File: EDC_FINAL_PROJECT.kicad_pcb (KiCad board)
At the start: 2 copper layers, 88.9 x 50.8 mm, 31 parts, among them J1 Screw_Terminal_01x02, J2 Screw_Terminal_01x03, SW1 SW_Push_DPDT, U1 LM317_TO-220, U2 LM337_TO220

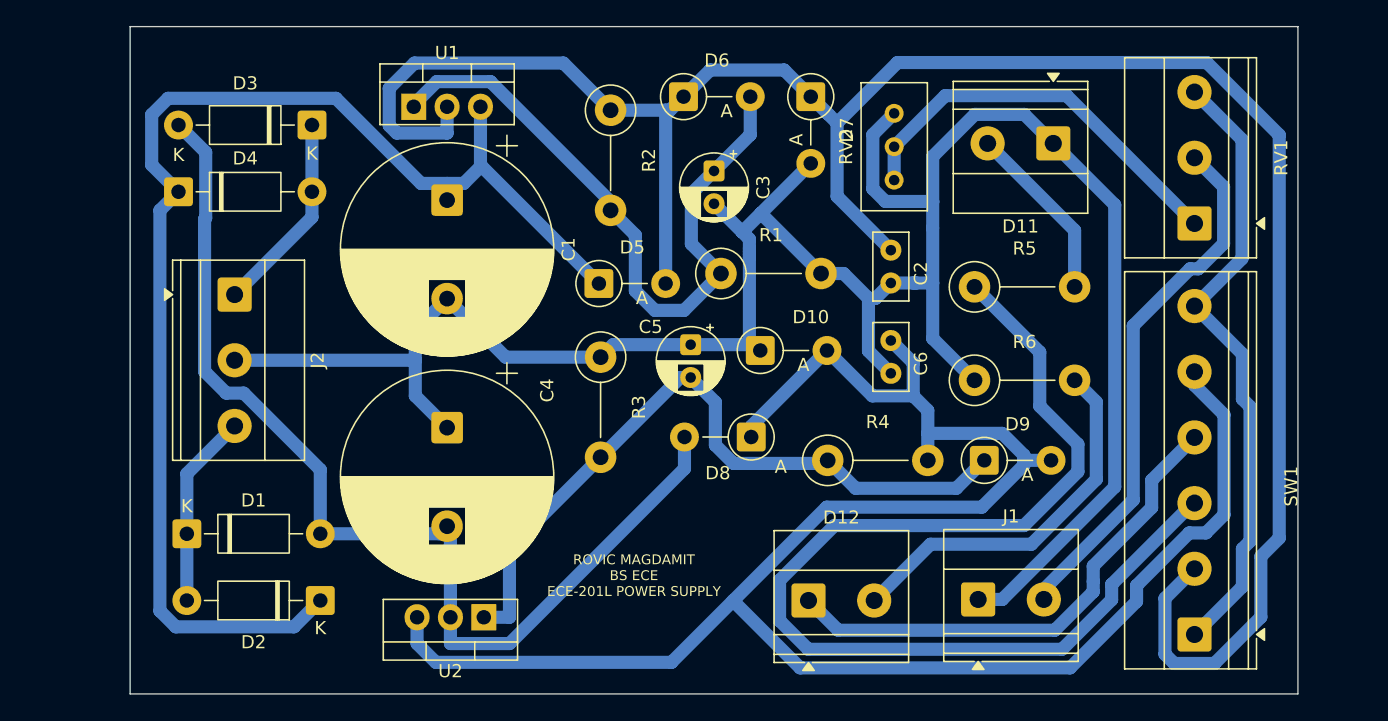
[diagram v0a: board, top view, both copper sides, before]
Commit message: 10.17.2025
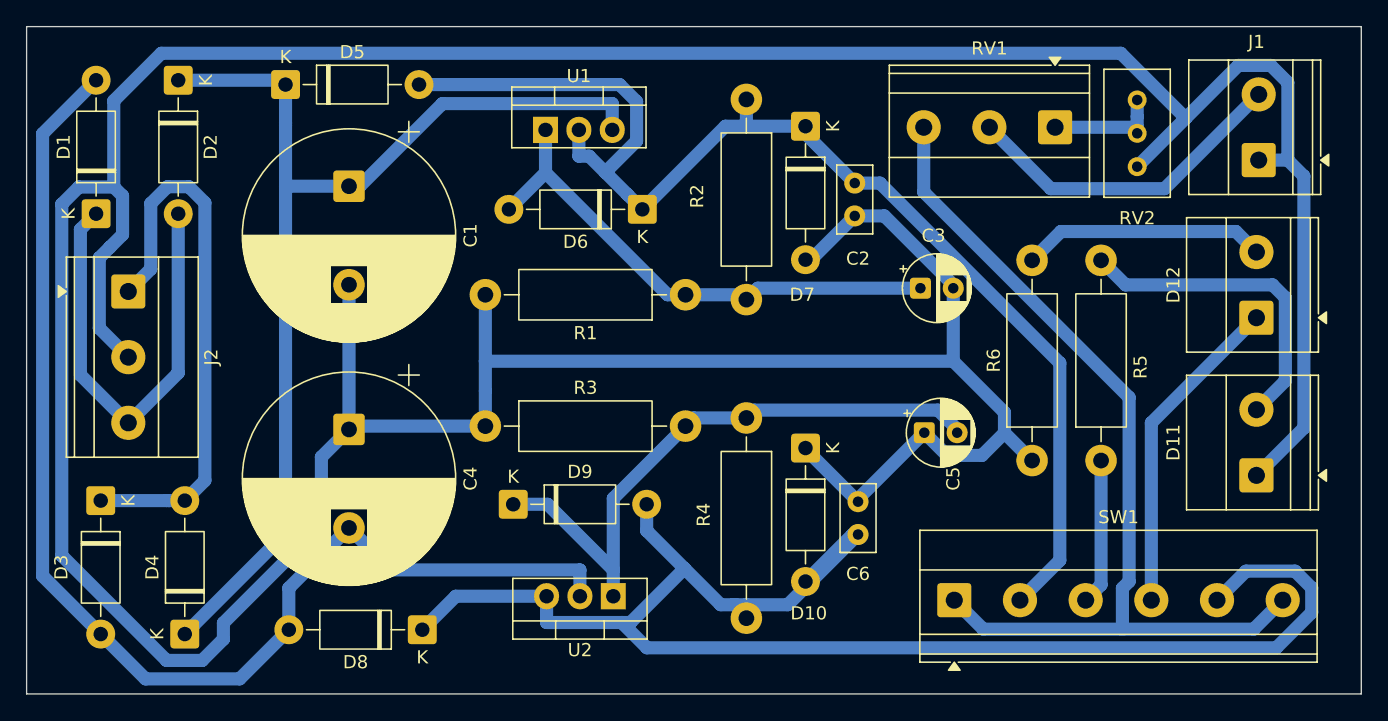
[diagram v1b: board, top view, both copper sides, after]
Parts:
- D10, D5, D6, D7, D8, D9: footprint Diode_THT:D_DO-41_SOD81_P5.08mm_Vertical_AnodeUp -> Diode_THT:D_DO-41_SOD81_P10.16mm_Horizontal
- R1, R2, R3, R4, R5, R6: footprint Resistor_THT:R_Axial_DIN0411_L9.9mm_D3.6mm_P7.62mm_Vertical -> Resistor_THT:R_Axial_DIN0411_L9.9mm_D3.6mm_P15.24mm_Horizontal
- moved D2 41.1 mm to (103.6, 77.2), turned to -90 degrees
- moved D12 40.3 mm to (185.7, 95.2), turned to 90 degrees
- moved J1 39.7 mm to (185.9, 83.2), turned to 90 degrees
- moved D9 36.0 mm to (129.1, 109.5)
- moved D4 33.7 mm to (104.1, 119.3), turned to 90 degrees
- moved D3 32.8 mm to (97.7, 109.2), turned to -90 degrees
- moved D11 29.6 mm to (185.7, 107.2), turned to 90 degrees
- moved D8 29.0 mm to (122.2, 119.0)
- moved D5 28.3 mm to (111.8, 77.5)
- moved D1 25.3 mm to (97.4, 87.3), turned to 90 degrees
- moved C5 19.0 mm to (160.4, 104.0), turned to 0 degrees
- moved RV2 18.9 mm to (176.6, 83.8), turned to -90 degrees
- moved SW1 18.5 mm to (162.7, 116.8), turned to 0 degrees
- moved C3 18.1 mm to (160.1, 93.0), turned to 0 degrees
- moved R5 16.4 mm to (173.9, 106.1), turned to 90 degrees
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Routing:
- net Net-(D10-K): track 176.9 -> 341.8 mm
- net Net-(R5-Pad1): track 84.3 -> 11.1 mm
- net Net-(D5-A): track 165.0 -> 95.5 mm
- net Net-(D10-A): track 149.9 -> 118.8 mm
- net Net-(D3-K): track 15.3 -> 42.3 mm
- net Net-(RV1-Pad3): track 47.8 -> 71.7 mm
- net Net-(RV1-Pad1): track 31.0 -> 8.79 mm
- net Net-(D1-K): track 14.8 -> 35.4 mm
- net Net-(D2-K): track 100.0 -> 82.8 mm
- net Net-(J1-Pin_2): track 40.6 -> 25.4 mm
- net Net-(D12-K): track 38.8 -> 24.8 mm
- net Net-(D1-A): track 81.1 -> 93.5 mm
- net Net-(D6-A): track 51.8 -> 40.1 mm
- net Net-(D11-A): track 13.7 -> 24.6 mm
- net Net-(D12-A): track 29.0 -> 18.6 mm
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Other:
- board size 88.9 x 50.8 mm -> 101.6 x 50.8 mm
- board text removed: "ROVIC MAGDAMIT BS ECE ECE-201L POWER SUPPLY"
